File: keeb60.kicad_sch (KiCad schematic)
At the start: 123 parts, among them K000 Esc, K001 1, K002 2, K003 3, K004 4, K005 5, K006 6, K007 7, K008 8, K009 9, K010 0, K011 _, K012 =, K013 Backspace, K100 Tab, K101 Q, K102 W, K103 E, K104 R, K105 T, K106 Y, K107 U, K108 I, K109 O, K110 P, K111 [, K112 ], K113 Pipe, K200 Caps Lock, K201 A, K202 S, K203 D, K204 F, K205 G, K206 H, K207 J, K208 K, K209 L, K210 ;, K211 ,, K213 Enter, K300 Shift, K302 Z, K303 X, K304 C, K305 V, K306 B, K307 N, K308 M, K309 ,, K310 ., K311 /, K313 Shift, K400 Ctrl, K401 Option, K402 Command, K406 Space, K410 Command, K411 Option, K412 Function, K413 Ctrl, U1 ProMicro

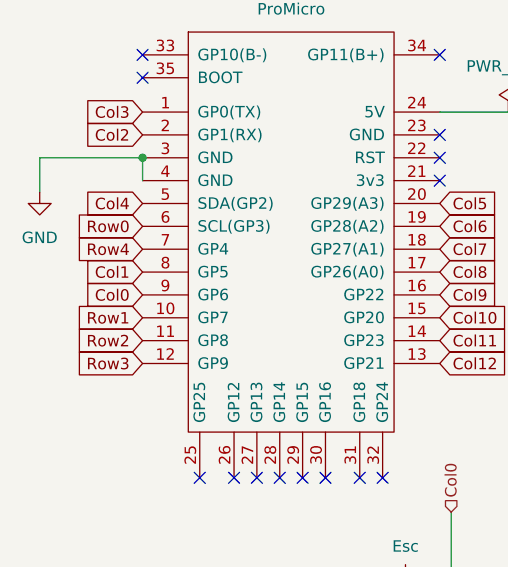
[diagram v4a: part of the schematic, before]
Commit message: V1.2
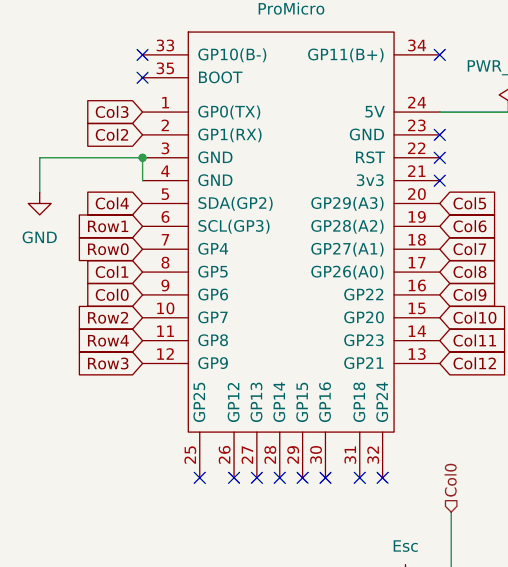
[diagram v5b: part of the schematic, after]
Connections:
- net Row0: now also U1.7 (GP4); no longer U1.6 (SCL(GP3))
- net Row1: now also U1.6 (SCL(GP3)); no longer U1.10 (GP7)
- net Row2: now also U1.10 (GP7); no longer U1.11 (GP8)
- net Row4: now also U1.11 (GP8); no longer U1.7 (GP4)
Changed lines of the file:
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@@
+		)
+	)
+	(global_label "Row4"
+		(shape input)
+		(at 27.94 55.88 180)
+		(fields_autoplaced yes)
+		(effects
+			(font
+				(size 1.27 1.27)
+			)
+			(justify right)
+		)
+		(property "Intersheetrefs" "${INTERSHEET_REFS}"
+			(at 19.9958 55.88 0)
+			(effects
+				(font
+					(size 1.27 1.27)
+				)
+				(justify right)
+				(hide yes)
+			)
 		)
 	)
@@
 		)
 	)
-	(global_label "Row4"
+	(global_label "Col4"
+		(shape input)
+		(at 27.94 40.64 180)
+		(fields_autoplaced yes)
+		(effects
+			(font
+				(size 1.27 1.27)
+			)
+			(justify right)
+		)
+		(property "Intersheetrefs" "${INTERSHEET_REFS}"
+			(at 20.6611 40.64 0)
+			(effects
+				(font
+					(size 1.27 1.27)
+				)
+				(justify right)
+				(hide yes)
+			)
+		)
+	)
+	(global_label "Col3"
+		(shape input)
+		(at 27.94 30.48 180)
+		(fields_autoplaced yes)
+		(effects
+			(font
+				(size 1.27 1.27)
+			)
+			(justify right)
+		)
+		(property "Intersheetrefs" "${INTERSHEET_REFS}"
+			(at 20.6611 30.48 0)
+			(effects
+				(font
+					(size 1.27 1.27)
+				)
+				(justify right)
+				(hide yes)
+			)
+		)
+	)
+	(global_label "Col11"
+		(shape input)
+		(at 60.96 55.88 0)
+		(fields_autoplaced yes)
+		(effects
+			(font
+				(size 1.27 1.27)
+			)
+			(justify left)
+		)
+		(property "Intersheetrefs" "${INTERSHEET_REFS}"
+			(at 69.4484 55.88 0)
+			(effects
+				(font
+					(size 1.27 1.27)
+				)
+				(justify left)
+				(hide yes)
+			)
+		)
+	)
+	(global_label "Row2"
+		(shape input)
+		(at 27.94 53.34 180)
+		(fields_autoplaced yes)
+		(effects
+			(font
+				(size 1.27 1.27)
+			)
+			(justify right)
+		)
+		(property "Intersheetrefs" "${INTERSHEET_REFS}"
+			(at 19.9958 53.34 0)
+			(effects
+				(font
+					(size 1.27 1.27)
+				)
+				(justify right)
+				(hide yes)
+			)
+		)
+	)
+	(global_label "Col10"
+		(shape input)
+		(at 60.96 53.34 0)
+		(fields_autoplaced yes)
+		(effects
+			(font
+				(size 1.27 1.27)
+			)
+			(justify left)
+		)
+		(property "Intersheetrefs" "${INTERSHEET_REFS}"
+			(at 69.4484 53.34 0)
+			(effects
+				(font
+					(size 1.27 1.27)
+				)
+				(justify left)
+				(hide yes)
+			)
+		)
+	)
+	(global_label "Col8"
+		(shape input)
+		(at 60.96 48.26 0)
+		(fields_autoplaced yes)
+		(effects
+			(font
+				(size 1.27 1.27)
+			)
+			(justify left)
+		)
+		(property "Intersheetrefs" "${INTERSHEET_REFS}"
+			(at 68.2389 48.26 0)
+			(effects
+				(font
+					(size 1.27 1.27)
+				)
+				(justify left)
+				(hide yes)
+			)
+		)
+	)
+	(global_label "Col6"
+		(shape input)
+		(at 60.96 43.18 0)
+		(fields_autoplaced yes)
+		(effects
+			(font
+				(size 1.27 1.27)
+			)
+			(justify left)
+		)
+		(property "Intersheetrefs" "${INTERSHEET_REFS}"
+			(at 68.2389 43.18 0)
+			(effects
+				(font
+					(size 1.27 1.27)
+				)
+				(justify left)
+				(hide yes)
+			)
+		)
+	)
+	(global_label "Row0"
 		(shape input)
 		(at 27.94 45.72 180)
@@
 		)
 	)
+	(global_label "Col0"
+		(shape input)
+		(at 27.94 50.8 180)
+		(fields_autoplaced yes)
+		(effects
+			(font
+				(size 1.27 1.27)
+			)
+			(justify right)
+		)
+		(property "Intersheetrefs" "${INTERSHEET_REFS}"
+			(at 20.6611 50.8 0)
+			(effects
+				(font
+					(size 1.27 1.27)
+				)
+				(justify right)
+				(hide yes)
+			)
+		)
+	)
 	(global_label "Row1"
 		(shape input)
-		(at 27.94 53.34 180)
-		(fields_autoplaced yes)
-		(effects
-			(font
-				(size 1.27 1.27)
-			)
-			(justify right)
-		)
-		(property "Intersheetrefs" "${INTERSHEET_REFS}"
-			(at 19.9958 53.34 0)
-			(effects
-				(font
-					(size 1.27 1.27)
-				)
-				(justify right)
-				(hide yes)
-			)
-		)
-	)
-	(global_label "Row2"
-		(shape input)
-		(at 27.94 55.88 180)
-		(fields_autoplaced yes)
-		(effects
-			(font
-				(size 1.27 1.27)
-			)
-			(justify right)
-		)
-		(property "Intersheetrefs" "${INTERSHEET_REFS}"
-			(at 19.9958 55.88 0)
-			(effects
-				(font
-					(size 1.27 1.27)
-				)
-				(justify right)
-				(hide yes)
-			)
-		)
-	)
-	(global_label "Col4"
-		(shape input)
-		(at 27.94 40.64 180)
-		(fields_autoplaced yes)
-		(effects
-			(font
-				(size 1.27 1.27)
-			)
-			(justify right)
-		)
-		(property "Intersheetrefs" "${INTERSHEET_REFS}"
-			(at 20.6611 40.64 0)
-			(effects
-				(font
-					(size 1.27 1.27)
-				)
-				(justify right)
-				(hide yes)
-			)
-		)
-	)
-	(global_label "Col3"
-		(shape input)
-		(at 27.94 30.48 180)
-		(fields_autoplaced yes)
-		(effects
-			(font
-				(size 1.27 1.27)
-			)
-			(justify right)
-		)
-		(property "Intersheetrefs" "${INTERSHEET_REFS}"
-			(at 20.6611 30.48 0)
-			(effects
-				(font
-					(size 1.27 1.27)
-				)
-				(justify right)
-				(hide yes)
-			)
-		)
-	)
-	(global_label "Col11"
-		(shape input)
-		(at 60.96 55.88 0)
-		(fields_autoplaced yes)
-		(effects
-			(font
-				(size 1.27 1.27)
-			)
-			(justify left)
-		)
-		(property "Intersheetrefs" "${INTERSHEET_REFS}"
-			(at 69.4484 55.88 0)
-			(effects
-				(font
-					(size 1.27 1.27)
-				)
-				(justify left)
-				(hide yes)
-			)
-		)
-	)
-	(global_label "Col10"
-		(shape input)
-		(at 60.96 53.34 0)
-		(fields_autoplaced yes)
-		(effects
-			(font
-				(size 1.27 1.27)
-			)
-			(justify left)
-		)
-		(property "Intersheetrefs" "${INTERSHEET_REFS}"
-			(at 69.4484 53.34 0)
-			(effects
-				(font
-					(size 1.27 1.27)
-				)
-				(justify left)
-				(hide yes)
-			)
-		)
-	)
-	(global_label "Col8"
-		(shape input)
-		(at 60.96 48.26 0)
-		(fields_autoplaced yes)
-		(effects
-			(font
-				(size 1.27 1.27)
-			)
-			(justify left)
-		)
-		(property "Intersheetrefs" "${INTERSHEET_REFS}"
-			(at 68.2389 48.26 0)
-			(effects
-				(font
-					(size 1.27 1.27)
-				)
-				(justify left)
-				(hide yes)
-			)
-		)
-	)
-	(global_label "Col6"
-		(shape input)
-		(at 60.96 43.18 0)
-		(fields_autoplaced yes)
-		(effects
-			(font
-				(size 1.27 1.27)
-			)
-			(justify left)
-		)
-		(property "Intersheetrefs" "${INTERSHEET_REFS}"
-			(at 68.2389 43.18 0)
-			(effects
-				(font
-					(size 1.27 1.27)
-				)
-				(justify left)
-				(hide yes)
-			)
-		)
-	)
-	(global_label "Row0"
-		(shape input)
 		(at 27.94 43.18 180)
 		(fields_autoplaced yes)
@@
 			(effects
 				(font
-					(size 1.27 1.27)
-				)
-				(justify right)
-				(hide yes)
-			)
-		)
-	)
-	(global_label "Col0"
-		(shape input)
-		(at 27.94 50.8 180)
-		(fields_autoplaced yes)
-		(effects
-			(font
-				(size 1.27 1.27)
-			)
-			(justify right)
-		)
-		(property "Intersheetrefs" "${INTERSHEET_REFS}"
-			(at 20.6611 50.8 0)
-			(effects
-				(font
